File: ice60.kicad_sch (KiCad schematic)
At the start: 31 parts, among them J1 SWD, J2 JST SH 4-pin, SW1 SW_Push, U1 RP2040, U2 W25Q128JVS, U3 XC6206PxxxMR-Regulator_Linear, U4 SRV05-4, Y1 12MHz

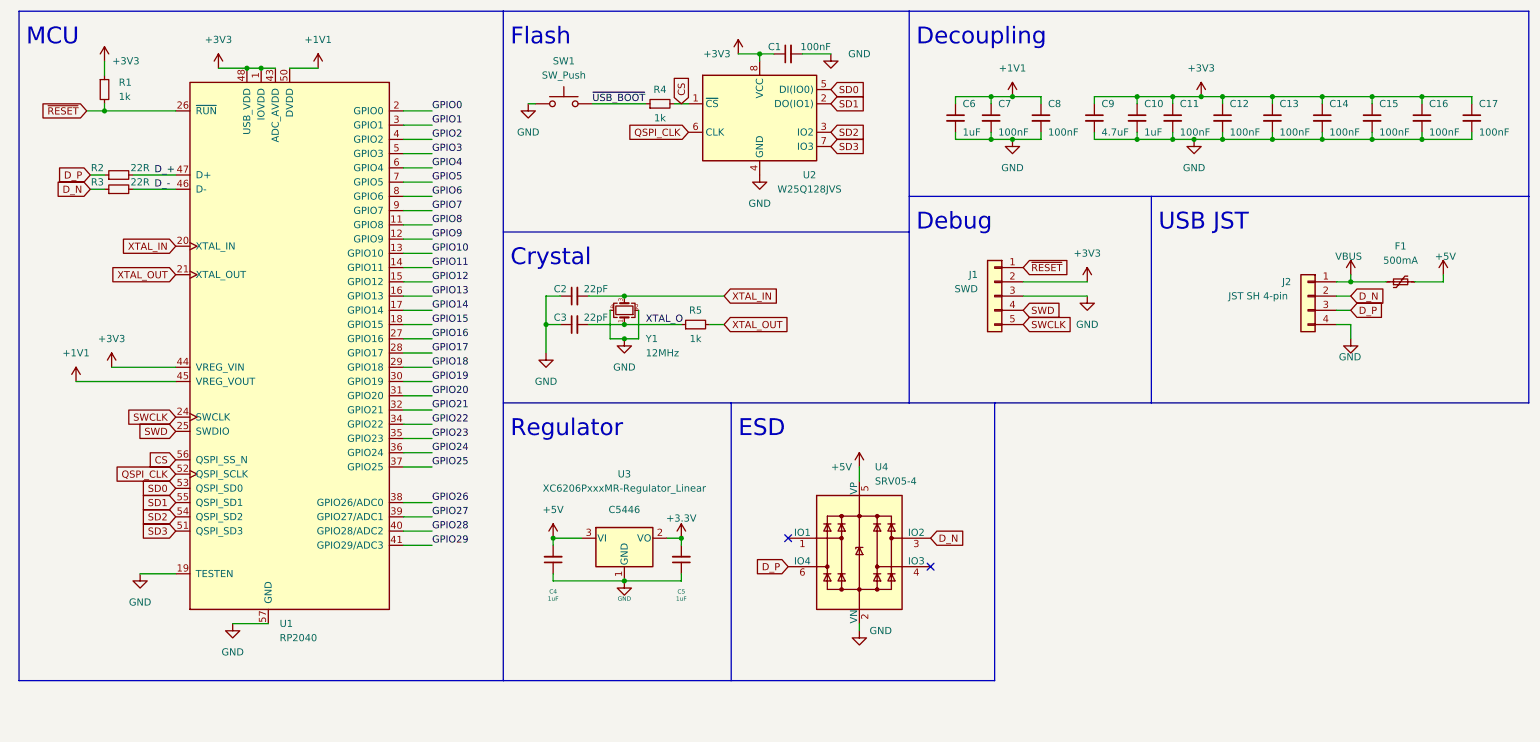
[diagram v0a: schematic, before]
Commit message: rearrange schematic
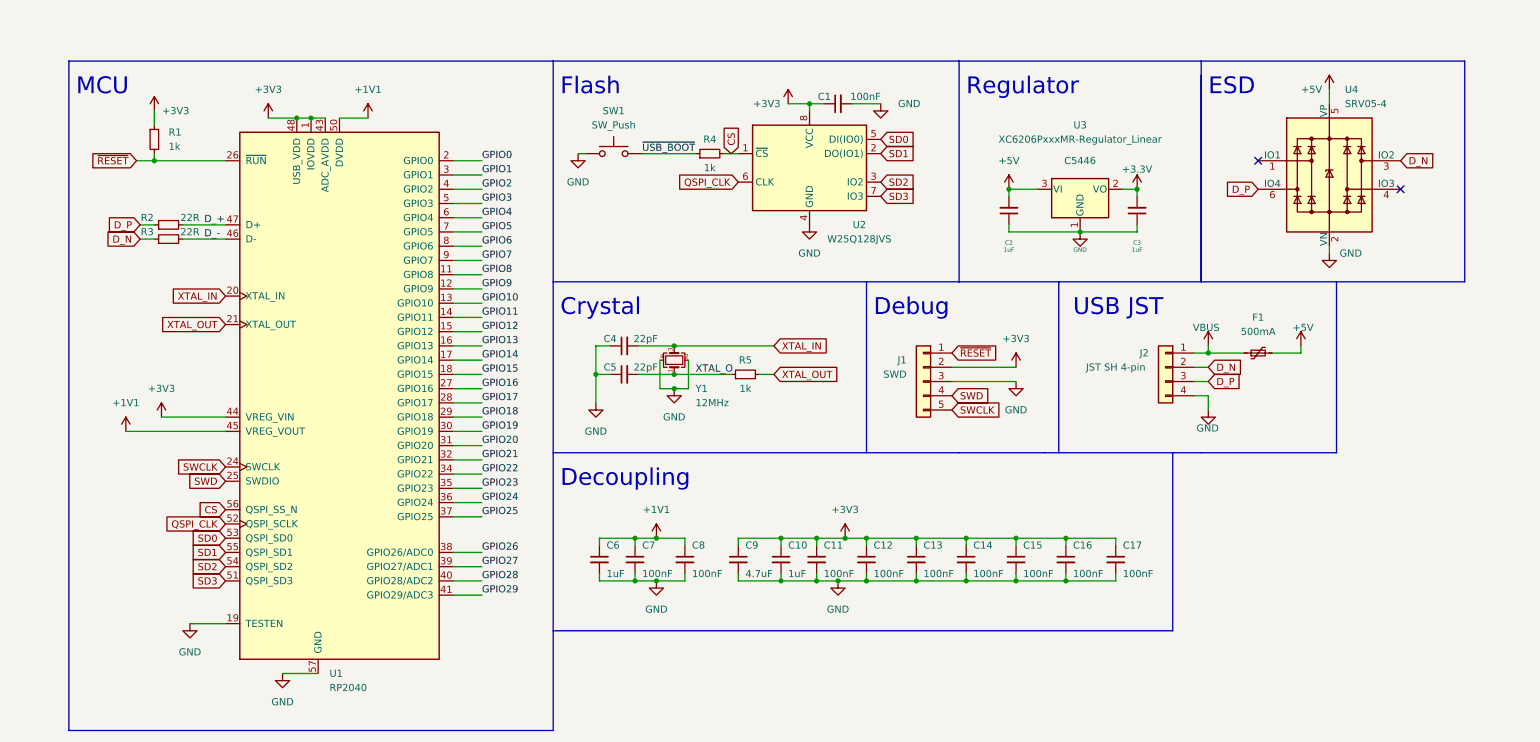
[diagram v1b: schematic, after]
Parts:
- renumbered C4 to C2, C5 to C3, C2 to C4, C3 to C5
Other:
- moved on the sheet: C1, C10, C11, C12, C13, C14, C15, C16, C17, C2, C3, C4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
